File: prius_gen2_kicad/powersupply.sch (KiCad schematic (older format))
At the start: 20 parts, among them U7 LMR14020, U8 AZ1117-3.3

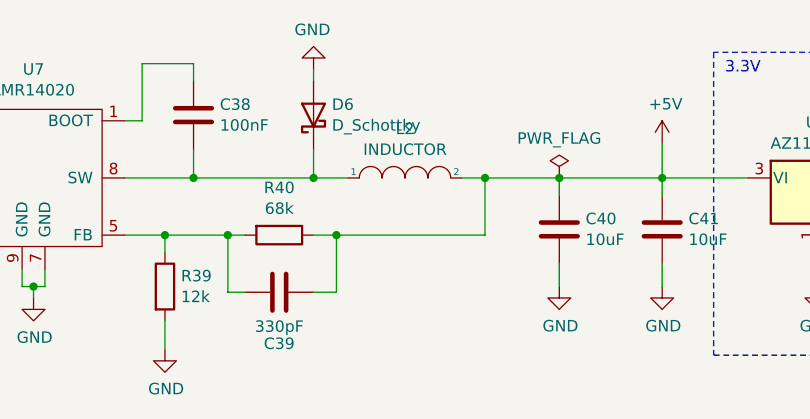
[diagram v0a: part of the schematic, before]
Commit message: started routing
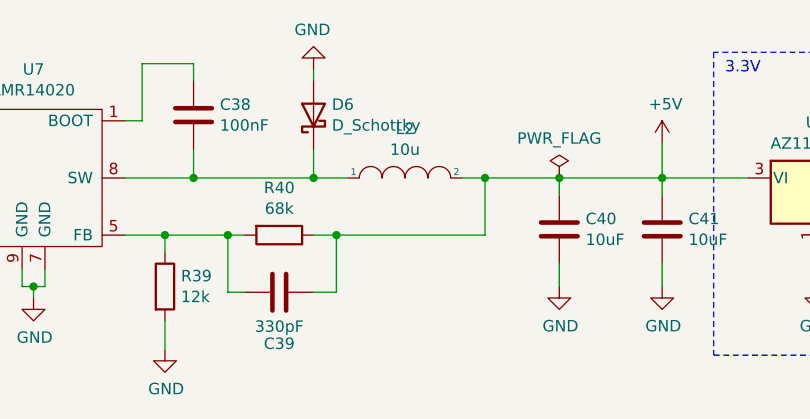
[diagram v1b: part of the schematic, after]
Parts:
- C34, C36, C37, C38, C39, C40, C41, C42: footprint (none) -> Capacitor_SMD:C_0603_1608Metric
- C35: footprint (none) -> Capacitor_THT:CP_Radial_D8.0mm_P3.50mm
- D4: footprint Diode_SMD:D_SOD-923 -> Diode_SMD:D_SMC
- D5, D6: footprint (none) -> Diode_SMD:D_SMA
- L1: footprint (none) -> Inductor_SMD:L_1210_3225Metric
- L2: value INDUCTOR -> 10u
- R37, R38, R39, R40: footprint (none) -> Resistor_SMD:R_0603_1608Metric
- U7: footprint (none) -> Package_SO:SOIC-8-1EP_3.9x4.9mm_P1.27mm_EP2.29x3mm
- U8: footprint (none) -> Package_TO_SOT_SMD:SOT-223-3_TabPin2
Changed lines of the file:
@@
 F 0 "U8" H 9250 3742 50  0000 C CNN
 F 1 "AZ1117-3.3" H 9250 3651 50  0000 C CNN
-F 2 "" H 9250 3750 50  0001 C CIN
+F 2 "Package_TO_SOT_SMD:SOT-223-3_TabPin2" H 9250 3750 50  0001 C CIN
 F 3 "https://www.diodes.com/assets/Datasheets/AZ1117.pdf" H 9250 3500 50  0001 C CNN
 	1    9250 3500
@@
 F 0 "D5" H 2600 3033 50  0000 C CNN
 F 1 "D_Schottky" H 2600 3124 50  0000 C CNN
-F 2 "" H 2600 3250 50  0001 C CNN
+F 2 "Diode_SMD:D_SMA" H 2600 3250 50  0001 C CNN
 F 3 "~" H 2600 3250 50  0001 C CNN
 	1    2600 3250
@@
 F 0 "D4" V 1954 3579 50  0000 L CNN
 F 1 "SM15T33CA" V 2045 3579 50  0000 L CNN
-F 2 "Diode_SMD:D_SOD-923" H 2000 3500 50  0001 C CNN
+F 2 "Diode_SMD:D_SMC" H 2000 3500 50  0001 C CNN
 F 3 "https://www.onsemi.com/pub/Collateral/ESD9B-D.PDF" H 2000 3500 50  0001 C CNN
 	1    2000 3500
@@
 F 0 "U7" H 5825 3875 50  0000 C CNN
 F 1 "LMR14020" H 5825 3784 50  0000 C CNN
-F 2 "" H 5725 3450 50  0001 C CNN
+F 2 "Package_SO:SOIC-8-1EP_3.9x4.9mm_P1.27mm_EP2.29x3mm" H 5725 3450 50  0001 C CNN
 F 3 "" H 5725 3450 50  0001 C CNN
 	1    5725 3450
@@
 F 0 "R37" H 3095 3496 50  0000 L CNN
 F 1 "1" H 3095 3405 50  0000 L CNN
-F 2 "" V 2955 3450 50  0001 C CNN
+F 2 "Resistor_SMD:R_0603_1608Metric" V 2955 3450 50  0001 C CNN
 F 3 "~" H 3025 3450 50  0001 C CNN
 	1    3025 3450
@@
 F 0 "C34" H 3140 3946 50  0000 L CNN
 F 1 "4.7uF" H 3140 3855 50  0000 L CNN
-F 2 "" H 3063 3750 50  0001 C CNN
+F 2 "Capacitor_SMD:C_0603_1608Metric" H 3063 3750 50  0001 C CNN
 F 3 "~" H 3025 3900 50  0001 C CNN
 	1    3025 3900
@@
 F 0 "L1" H 3600 3465 50  0000 C CNN
 F 1 "2.2uH" H 3600 3374 50  0000 C CNN
-F 2 "" H 3600 3250 50  0001 C CNN
+F 2 "Inductor_SMD:L_1210_3225Metric" H 3600 3250 50  0001 C CNN
 F 3 "~" H 3600 3250 50  0001 C CNN
 	1    3600 3250
@@
 F 0 "C35" H 4218 3571 50  0000 L CNN
 F 1 "56uF" H 4218 3480 50  0000 L CNN
-F 2 "" H 4138 3375 50  0001 C CNN
+F 2 "Capacitor_THT:CP_Radial_D8.0mm_P3.50mm" H 4138 3375 50  0001 C CNN
 F 3 "~" H 4100 3525 50  0001 C CNN
 	1    4100 3525
@@
 F 0 "C36" H 4690 3571 50  0000 L CNN
 F 1 "1uF" H 4690 3480 50  0000 L CNN
-F 2 "" H 4613 3375 50  0001 C CNN
+F 2 "Capacitor_SMD:C_0603_1608Metric" H 4613 3375 50  0001 C CNN
 F 3 "~" H 4575 3525 50  0001 C CNN
 	1    4575 3525
@@
 F 0 "R38" H 5095 3846 50  0000 L CNN
 F 1 "10k" H 5095 3755 50  0000 L CNN
-F 2 "" V 4955 3800 50  0001 C CNN
+F 2 "Resistor_SMD:R_0603_1608Metric" V 4955 3800 50  0001 C CNN
 F 3 "~" H 5025 3800 50  0001 C CNN
 	1    5025 3800
@@
 F 0 "C37" H 5465 4021 50  0000 L CNN
 F 1 "10nF" H 5465 3930 50  0000 L CNN
-F 2 "" H 5388 3825 50  0001 C CNN
+F 2 "Capacitor_SMD:C_0603_1608Metric" H 5388 3825 50  0001 C CNN
 F 3 "~" H 5350 3975 50  0001 C CNN
 	1    5350 3975
@@
 F 0 "C38" H 6640 3271 50  0000 L CNN
 F 1 "100nF" H 6640 3180 50  0000 L CNN
-F 2 "" H 6563 3075 50  0001 C CNN
+F 2 "Capacitor_SMD:C_0603_1608Metric" H 6563 3075 50  0001 C CNN
 F 3 "~" H 6525 3225 50  0001 C CNN
 	1    6525 3225
@@
 F 0 "D6" V 7096 3145 50  0000 R CNN
 F 1 "D_Schottky" V 7005 3145 50  0000 R CNN
-F 2 "" H 7050 3225 50  0001 C CNN
+F 2 "Diode_SMD:D_SMA" H 7050 3225 50  0001 C CNN
 F 3 "~" H 7050 3225 50  0001 C CNN
 	1    7050 3225
@@
 P 7450 3500
 F 0 "L2" H 7450 3715 50  0000 C CNN
-F 1 "INDUCTOR" H 7450 3624 50  0000 C CNN
+F 1 "10u" H 7450 3624 50  0000 C CNN
 F 2 "" H 7450 3500 50  0001 C CNN
 F 3 "~" H 7450 3500 50  0001 C CNN
@@
 F 0 "R39" H 6470 4021 50  0000 L CNN
 F 1 "12k" H 6470 3930 50  0000 L CNN
-F 2 "" V 6330 3975 50  0001 C CNN
+F 2 "Resistor_SMD:R_0603_1608Metric" V 6330 3975 50  0001 C CNN
 F 3 "~" H 6400 3975 50  0001 C CNN
 	1    6400 3975
@@
 F 0 "R40" V 6693 3750 50  0000 C CNN
 F 1 "68k" V 6784 3750 50  0000 C CNN
-F 2 "" V 6830 3750 50  0001 C CNN
+F 2 "Resistor_SMD:R_0603_1608Metric" V 6830 3750 50  0001 C CNN
 F 3 "~" H 6900 3750 50  0001 C CNN
 	1    6900 3750
@@
 F 0 "C39" V 6675 4000 50  0000 C CNN
 F 1 "330pF" V 6750 4000 50  0000 C CNN
-F 2 "" H 6938 3850 50  0001 C CNN
+F 2 "Capacitor_SMD:C_0603_1608Metric" H 6938 3850 50  0001 C CNN
 F 3 "~" H 6900 4000 50  0001 C CNN
 	1    6900 4000
@@
 F 0 "C40" H 8240 3771 50  0000 L CNN
 F 1 "10uF" H 8240 3680 50  0000 L CNN
-F 2 "" H 8163 3575 50  0001 C CNN
+F 2 "Capacitor_SMD:C_0603_1608Metric" H 8163 3575 50  0001 C CNN
 F 3 "~" H 8125 3725 50  0001 C CNN
 	1    8125 3725
@@
 F 0 "C41" H 8690 3771 50  0000 L CNN
 F 1 "10uF" H 8690 3680 50  0000 L CNN
-F 2 "" H 8613 3575 50  0001 C CNN
+F 2 "Capacitor_SMD:C_0603_1608Metric" H 8613 3575 50  0001 C CNN
 F 3 "~" H 8575 3725 50  0001 C CNN
 	1    8575 3725
@@
 F 0 "C42" H 9990 3771 50  0000 L CNN
 F 1 "4.7uF" H 9990 3680 50  0000 L CNN
-F 2 "" H 9913 3575 50  0001 C CNN
+F 2 "Capacitor_SMD:C_0603_1608Metric" H 9913 3575 50  0001 C CNN
 F 3 "~" H 9875 3725 50  0001 C CNN
 	1    9875 3725

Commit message: cam and more...
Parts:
- L2: footprint (none) -> prius_gen2_kicad:MWSA0503
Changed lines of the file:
@@
 F 0 "L2" H 7450 3715 50  0000 C CNN
 F 1 "10u" H 7450 3624 50  0000 C CNN
-F 2 "" H 7450 3500 50  0001 C CNN
+F 2 "prius_gen2_kicad:MWSA0503" H 7450 3500 50  0001 C CNN
 F 3 "~" H 7450 3500 50  0001 C CNN
 	1    7450 3500
